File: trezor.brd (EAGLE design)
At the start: 50 x 26.7 mm, 27 parts, among them IC1 MCP1703CB, Q2 16MHz, U1 STM32F205RET6, U2 USB, U3 DISPLAY

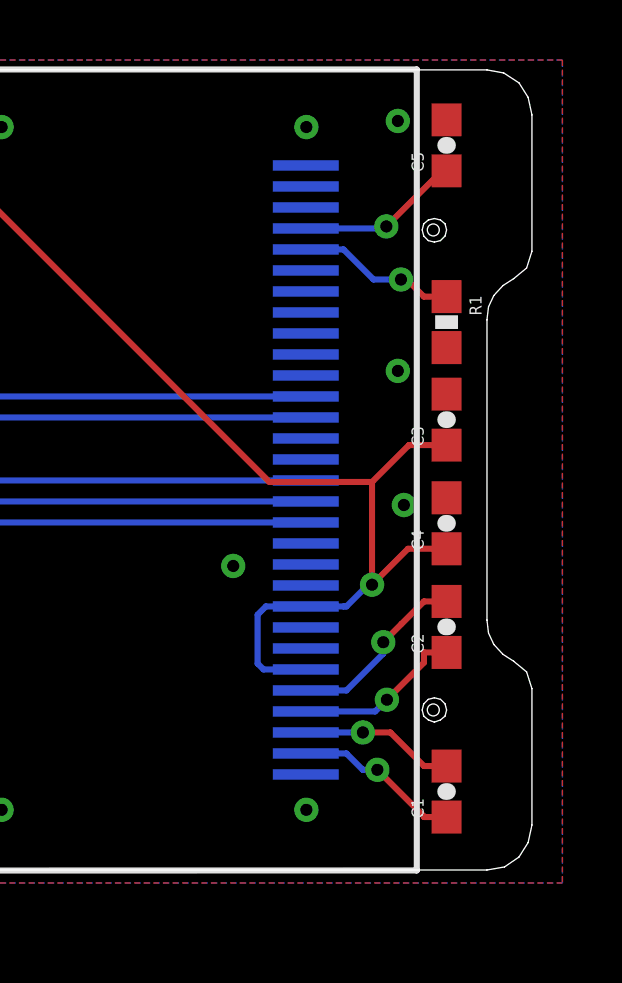
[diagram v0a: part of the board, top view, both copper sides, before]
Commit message: move capacitors to the edge
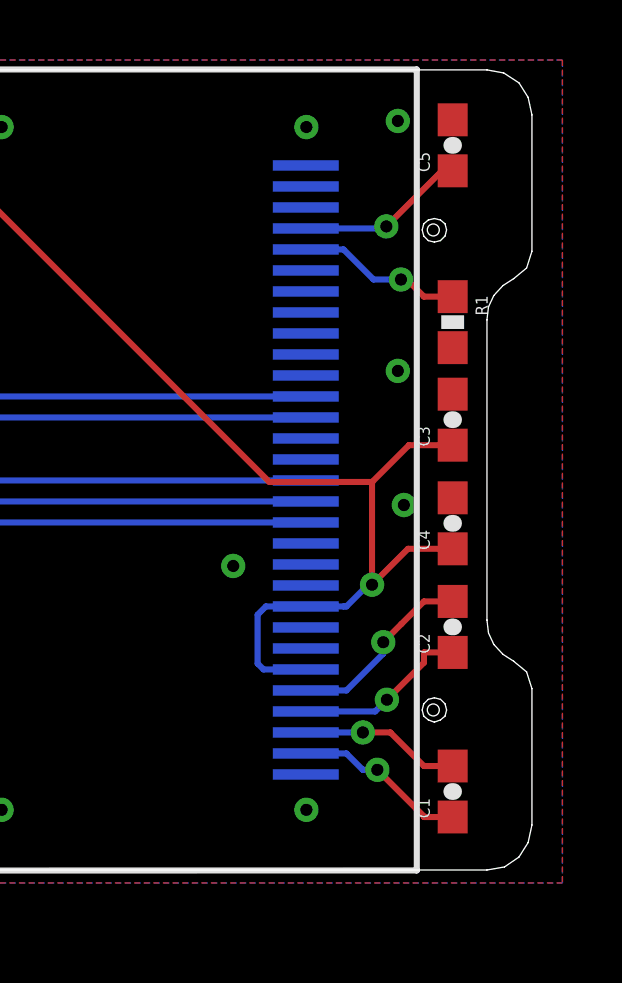
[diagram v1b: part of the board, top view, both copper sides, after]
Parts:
- moved C1 0.20 mm to (47.3, 2.64)
- moved C2 0.20 mm to (47.3, 8.13)
- moved C3 0.20 mm to (47.3, 15.0)
- moved C4 0.20 mm to (47.3, 11.6)
- moved C5 0.20 mm to (47.3, 24.2)
- moved R1 0.20 mm to (47.3, 18.3)
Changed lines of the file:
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@@
 </element>
 <element name="U3" library="microbuilder" package="UG-2864HSWEG01_0.96IN_WRAPAROUND" value="DISPLAY" x="41.2496" y="13.3604" rot="R90"/>
-<element name="C1" library="SparkFun-Passives" package="0603-CAP" value="1uF" x="47.1424" y="2.6416" rot="R90"/>
-<element name="C2" library="SparkFun-Passives" package="0603-CAP" value="1uF" x="47.1424" y="8.128" rot="R90"/>
-<element name="C3" library="SparkFun-Passives" package="0603-CAP" value="0.1uF" x="47.1424" y="15.0368" rot="R90"/>
-<element name="C4" library="SparkFun-Passives" package="0603-CAP" value="1uF" x="47.1424" y="11.5824" rot="R90"/>
-<element name="C5" library="SparkFun-Passives" package="0603-CAP" value="2.2uF" x="47.1424" y="24.1808" rot="R90"/>
-<element name="R1" library="SparkFun-Passives" package="0603-RES" value="390k" x="47.1424" y="18.288" rot="R270"/>
+<element name="C1" library="SparkFun-Passives" package="0603-CAP" value="1uF" x="47.3456" y="2.6416" rot="R90"/>
+<element name="C2" library="SparkFun-Passives" package="0603-CAP" value="1uF" x="47.3456" y="8.128" rot="R90"/>
+<element name="C3" library="SparkFun-Passives" package="0603-CAP" value="0.1uF" x="47.3456" y="15.0368" rot="R90"/>
+<element name="C4" library="SparkFun-Passives" package="0603-CAP" value="1uF" x="47.3456" y="11.5824" rot="R90"/>
+<element name="C5" library="SparkFun-Passives" package="0603-CAP" value="2.2uF" x="47.3456" y="24.1808" rot="R90"/>
+<element name="R1" library="SparkFun-Passives" package="0603-RES" value="390k" x="47.3456" y="18.288" rot="R270"/>
 <element name="S1" library="SparkFun-Electromechanical" package="TACTILE_SWITCH_SMD" value="SWITCH-MOMENTARY-2SMD" x="23.876" y="20.6248" rot="R270"/>
 <element name="S2" library="SparkFun-Electromechanical" package="TACTILE_SWITCH_SMD" value="SWITCH-MOMENTARY-2SMD" x="23.876" y="6.096" rot="R270"/>
@@
 <wire x1="15.2772" y1="21.7424" x2="15.2772" y2="22.9616" width="0.2032" layer="1"/>
 <wire x1="15.2772" y1="22.9616" x2="14.4644" y2="23.7744" width="0.2032" layer="1"/>
-<wire x1="47.1424" y1="10.7324" x2="45.8551" y2="10.7324" width="0.2032" layer="1"/>
+<wire x1="47.3456" y1="10.7324" x2="45.8551" y2="10.7324" width="0.2032" layer="1"/>
 <wire x1="24.8231" y1="26.0042" x2="28.1899" y2="26.0042" width="0.2032" layer="1"/>
-<wire x1="47.1424" y1="14.1868" x2="45.886" y2="14.1868" width="0.2032" layer="1"/>
+<wire x1="47.3456" y1="14.1868" x2="45.886" y2="14.1868" width="0.2032" layer="1"/>
 <wire x1="44.6584" y1="9.5357" x2="44.6584" y2="12.9592" width="0.2032" layer="1"/>
 <wire x1="44.6584" y1="12.9592" x2="45.886" y2="14.1868" width="0.2032" layer="1"/>
@@
 <contactref element="C1" pad="1"/>
 <wire x1="42.4496" y1="3.9104" x2="43.8037" y2="3.9104" width="0.2032" layer="16"/>
-<wire x1="47.1424" y1="1.7916" x2="46.3883" y2="1.7916" width="0.2032" layer="1"/>
+<wire x1="47.3456" y1="1.7916" x2="46.3883" y2="1.7916" width="0.2032" layer="1"/>
 <wire x1="44.8347" y1="3.3656" x2="46.3883" y2="1.812" width="0.2032" layer="1"/>
 <wire x1="46.3883" y1="1.812" x2="46.3883" y2="1.7916" width="0.2032" layer="1"/>
@@
 <contactref element="U3" pad="4"/>
 <contactref element="C2" pad="1"/>
-<wire x1="47.1424" y1="7.278" x2="46.3883" y2="7.278" width="0.2032" layer="1"/>
+<wire x1="47.3456" y1="7.278" x2="46.3883" y2="7.278" width="0.2032" layer="1"/>
 <wire x1="45.1528" y1="5.7014" x2="46.3883" y2="6.9369" width="0.2032" layer="1"/>
 <wire x1="46.3883" y1="6.9369" x2="46.3883" y2="7.278" width="0.2032" layer="1"/>
@@
 <contactref element="U3" pad="3"/>
 <contactref element="C1" pad="2"/>
-<wire x1="47.1424" y1="3.4916" x2="46.3883" y2="3.4916" width="0.2032" layer="1"/>
+<wire x1="47.3456" y1="3.4916" x2="46.3883" y2="3.4916" width="0.2032" layer="1"/>
 <wire x1="44.3512" y1="4.6104" x2="45.2695" y2="4.6104" width="0.2032" layer="1"/>
 <wire x1="45.2695" y1="4.6104" x2="46.3883" y2="3.4916" width="0.2032" layer="1"/>
@@
 <contactref element="C2" pad="2"/>
 <wire x1="42.4496" y1="6.0104" x2="43.8037" y2="6.0104" width="0.2032" layer="16"/>
-<wire x1="47.1424" y1="8.978" x2="46.3883" y2="8.978" width="0.2032" layer="1"/>
+<wire x1="47.3456" y1="8.978" x2="46.3883" y2="8.978" width="0.2032" layer="1"/>
 <wire x1="45.0324" y1="7.618" x2="45.6379" y2="8.2276" width="0.2032" layer="1"/>
 <wire x1="45.6379" y1="8.2276" x2="46.3883" y2="8.978" width="0.2032" layer="1"/>
@@
 <wire x1="42.4496" y1="21.4104" x2="45.0659" y2="21.4104" width="0.2032" layer="16"/>
 <wire x1="45.0659" y1="21.4104" x2="45.1344" y2="21.4789" width="0.2032" layer="16"/>
-<wire x1="47.1424" y1="23.3308" x2="46.9863" y2="23.3308" width="0.2032" layer="1"/>
+<wire x1="47.3456" y1="23.3308" x2="46.9863" y2="23.3308" width="0.2032" layer="1"/>
 <wire x1="46.9863" y1="23.3308" x2="45.1344" y2="21.4789" width="0.2032" layer="1"/>
 </signal>
@@
 <contactref element="U3" pad="26"/>
 <contactref element="R1" pad="1"/>
-<wire x1="47.1424" y1="19.138" x2="46.3883" y2="19.138" width="0.2032" layer="1"/>
+<wire x1="47.3456" y1="19.138" x2="46.3883" y2="19.138" width="0.2032" layer="1"/>
 <wire x1="45.6209" y1="19.7087" x2="45.8176" y2="19.7087" width="0.2032" layer="1"/>
 <wire x1="45.8176" y1="19.7087" x2="46.3883" y2="19.138" width="0.2032" layer="1"/>

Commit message: add items to trezor bom
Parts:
- C12, C13, C14, C15, C16: value 100nF -> 0.1uF
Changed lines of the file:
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@@
 <element name="C10" library="SparkFun-Passives" package="0603-CAP" value="1uF" x="5.08" y="18.288"/>
 <element name="C11" library="SparkFun-Passives" package="0603-CAP" value="1uF" x="10.668" y="6.5024" rot="R270"/>
-<element name="C13" library="SparkFun-Passives" package="0603-CAP" value="100nF" x="6.9088" y="12.3952" rot="R270"/>
-<element name="C12" library="SparkFun-Passives" package="0603-CAP" value="100nF" x="25.6032" y="13.3604" rot="R270"/>
-<element name="C15" library="SparkFun-Passives" package="0603-CAP" value="100nF" x="24.1808" y="10.5664"/>
-<element name="C16" library="SparkFun-Passives" package="0603-CAP" value="100nF" x="13.6144" y="23.7744"/>
-<element name="C14" library="SparkFun-Passives" package="0603-CAP" value="100nF" x="14.4272" y="21.7424"/>
+<element name="C13" library="SparkFun-Passives" package="0603-CAP" value="0.1uF" x="6.9088" y="12.3952" rot="R270"/>
+<element name="C12" library="SparkFun-Passives" package="0603-CAP" value="0.1uF" x="25.6032" y="13.3604" rot="R270"/>
+<element name="C15" library="SparkFun-Passives" package="0603-CAP" value="0.1uF" x="24.1808" y="10.5664"/>
+<element name="C16" library="SparkFun-Passives" package="0603-CAP" value="0.1uF" x="13.6144" y="23.7744"/>
+<element name="C14" library="SparkFun-Passives" package="0603-CAP" value="0.1uF" x="14.4272" y="21.7424"/>
 <element name="C17" library="SparkFun-Passives" package="0603-CAP" value="2.2uF" x="23.5712" y="13.3604" rot="R270"/>
 <element name="IC1" library="linear" package="SOT23" value="MCP1703CB" x="7.112" y="8.7376" rot="R90"/>
